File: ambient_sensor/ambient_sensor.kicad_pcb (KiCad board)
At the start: 2 copper layers, 69.5 x 54 mm, 22 parts, among them J1 Conn_01x02_Pin, J2 Conn_01x02_Pin, J3 Conn_01x05_Pin, J4 Conn_01x01_Pin, J5 Conn_01x04_Pin, J6 Conn_01x02_Pin, U4 ATmega328-P, U6 LD1117S33TR_SOT223, Y1 Crystal

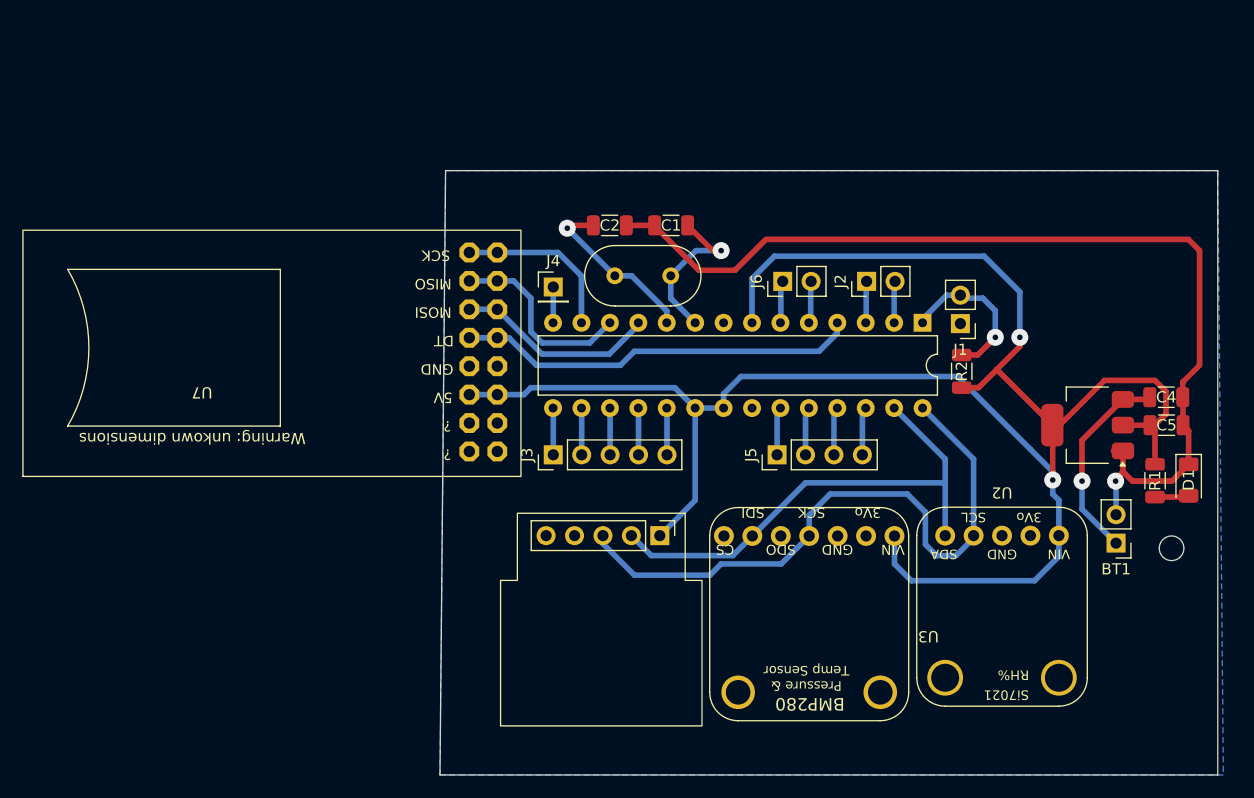
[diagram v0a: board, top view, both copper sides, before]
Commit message: almost all warnings
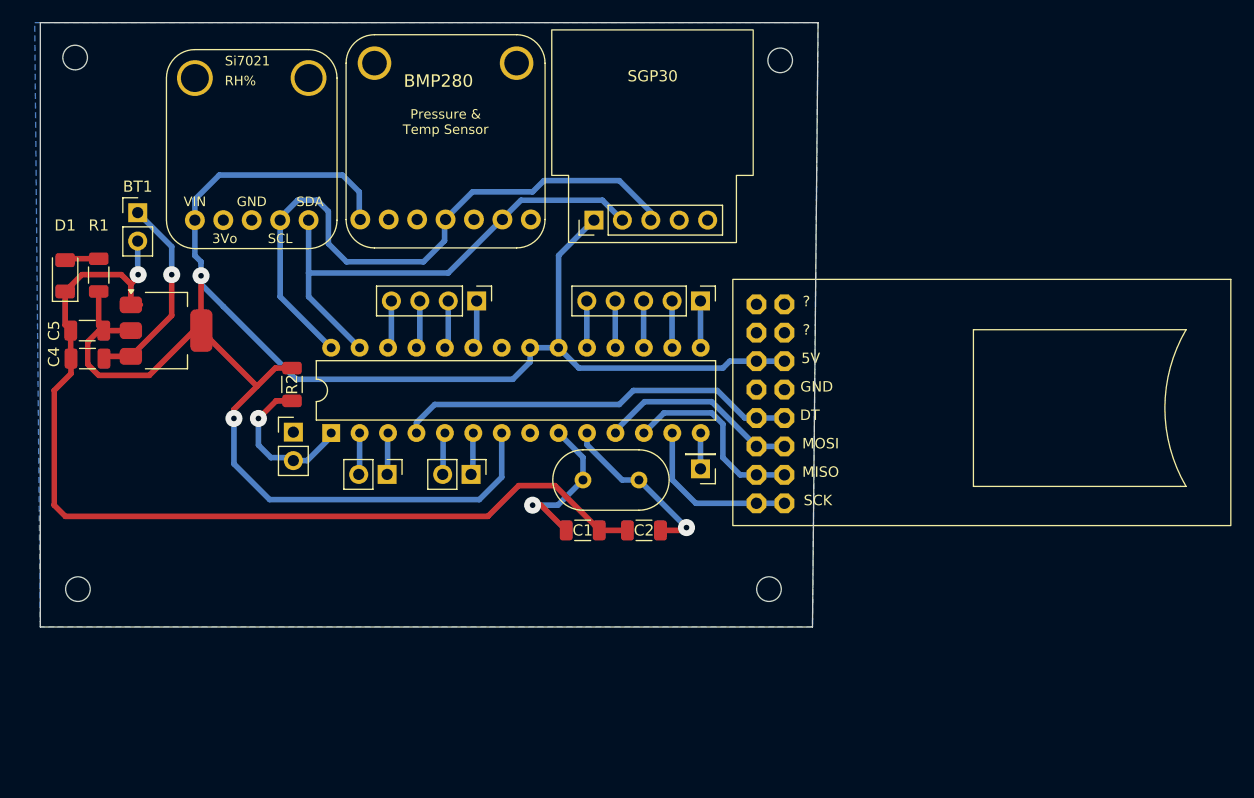
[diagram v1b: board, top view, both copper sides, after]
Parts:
- added REF**: MountingHole_2.2mm_M2, MountingHole:MountingHole_2.2mm_M2, F.Cu at (227.9, 141.8)
- added REF**: MountingHole_2.2mm_M2, MountingHole:MountingHole_2.2mm_M2, F.Cu at (166.1, 141.8)
- added REF**: MountingHole_2.2mm_M2, MountingHole:MountingHole_2.2mm_M2, F.Cu at (228.9, 94.5)
- moved U7 116.0 mm to (271.2, 138.1), turned to 0 degrees
- moved REF** 107.3 mm to (165.9, 94.2), turned to 180 degrees
- moved D1 102.0 mm to (165.0, 113.8), turned to 90 degrees
- moved C5 96.8 mm to (167.0, 118.7), turned to 0 degrees
- moved C4 96.5 mm to (167.0, 121.2), turned to 0 degrees
- moved R1 96.2 mm to (168.0, 113.7), turned to 90 degrees
- moved BT1 92.3 mm to (171.5, 108.1), turned to 0 degrees
- moved U6 82.8 mm to (174.0, 118.7), turned to 0 degrees
- moved U2 69.8 mm to (181.7, 113.1), turned to 0 degrees
- moved J1 60.4 mm to (185.4, 127.7), turned to 0 degrees
- moved R2 59.9 mm to (185.3, 123.5), turned to 90 degrees
- moved U1 56.2 mm to (220.5, 95.3), turned to 180 degrees
- moved U4 53.8 mm to (188.8, 127.8), turned to 90 degrees
- moved J2 46.2 mm to (193.8, 131.5), turned to -90 degrees
- moved U3 36.7 mm to (198.8, 113.3), turned to 0 degrees
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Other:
- outline, holes or cut-outs redrawn
- board text added: "SGP30"
